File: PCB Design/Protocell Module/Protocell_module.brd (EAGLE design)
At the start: 70.8 x 27.9 mm, 19 parts, among them IC1 MC7805BDTRKG, X3 RJ45-8X

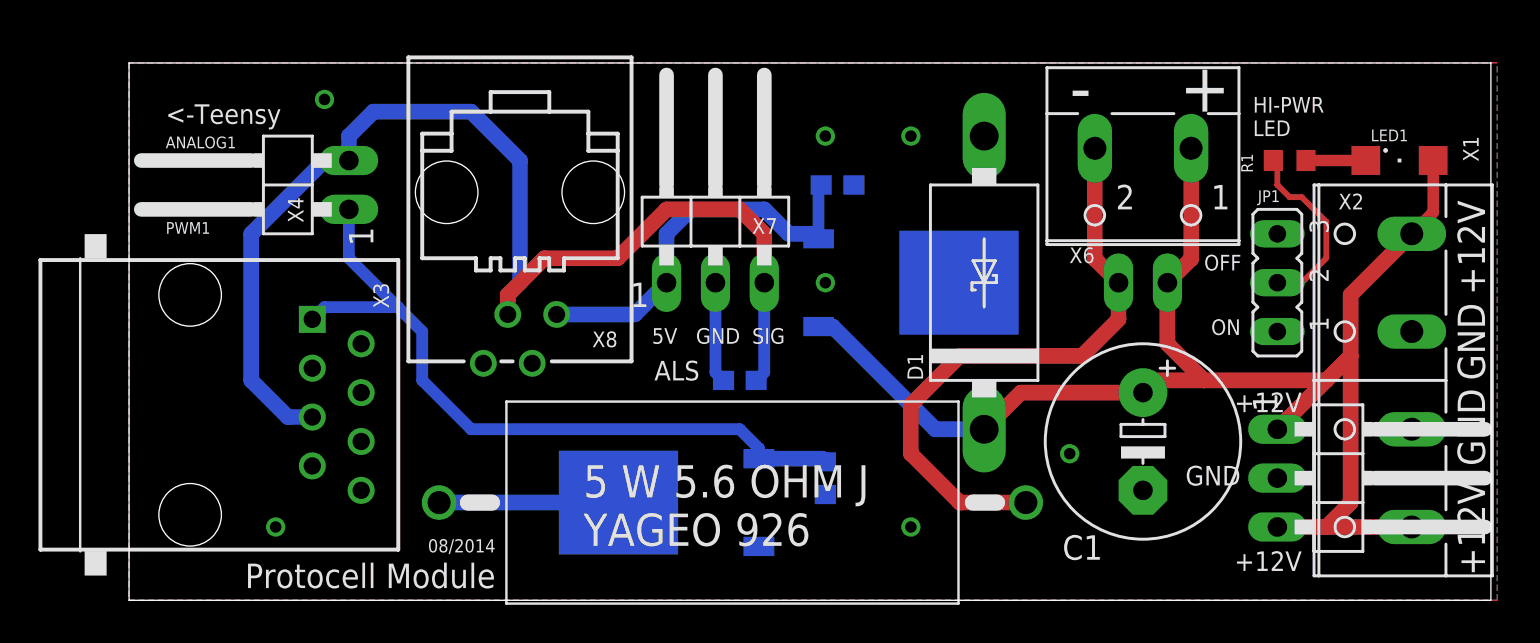
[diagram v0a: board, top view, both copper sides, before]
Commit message: Generated gerber files
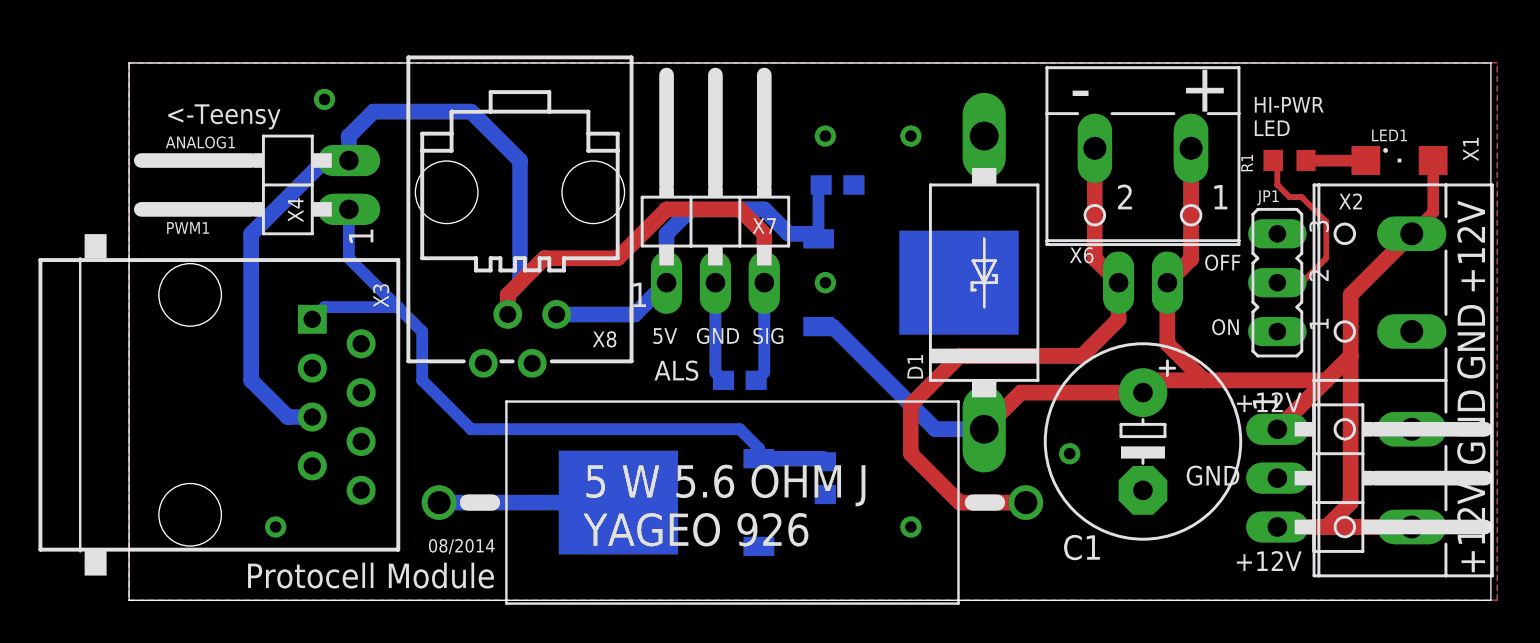
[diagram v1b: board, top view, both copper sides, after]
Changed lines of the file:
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@@
 </class>
 </classes>
-<designrules name="default *">
-<description language="de">&lt;b&gt;EAGLE Design Rules&lt;/b&gt;
-&lt;p&gt;
-Die Standard-Design-Rules sind so gewählt, dass sie für
-die meisten Anwendungen passen. Sollte ihre Platine
-besondere Anforderungen haben, treffen Sie die erforderlichen
-Einstellungen hier und speichern die Design Rules unter
-einem neuen Namen ab.</description>
+<designrules name="SparkFun">
 <description language="en">&lt;b&gt;EAGLE Design Rules&lt;/b&gt;
 &lt;p&gt;
@@
 <param name="mtCopper" value="0.035mm 0.035mm 0.035mm 0.035mm 0.035mm 0.035mm 0.035mm 0.035mm 0.035mm 0.035mm 0.035mm 0.035mm 0.035mm 0.035mm 0.035mm 0.035mm"/>
 <param name="mtIsolate" value="1.5mm 0.15mm 0.2mm 0.15mm 0.2mm 0.15mm 0.2mm 0.15mm 0.2mm 0.15mm 0.2mm 0.15mm 0.2mm 0.15mm 0.2mm"/>
-<param name="mdWireWire" value="10mil"/>
-<param name="mdWirePad" value="10mil"/>
-<param name="mdWireVia" value="10mil"/>
-<param name="mdPadPad" value="10mil"/>
-<param name="mdPadVia" value="10mil"/>
-<param name="mdViaVia" value="10mil"/>
+<param name="mdWireWire" value="8mil"/>
+<param name="mdWirePad" value="8mil"/>
+<param name="mdWireVia" value="8mil"/>
+<param name="mdPadPad" value="8mil"/>
+<param name="mdPadVia" value="8mil"/>
+<param name="mdViaVia" value="8mil"/>
 <param name="mdSmdPad" value="8mil"/>
 <param name="mdSmdVia" value="8mil"/>
@@
 <param name="mdViaViaSameLayer" value="8mil"/>
 <param name="mnLayersViaInSmd" value="2"/>
-<param name="mdCopperDimension" value="40mil"/>
+<param name="mdCopperDimension" value="10mil"/>
 <param name="mdDrill" value="8mil"/>
 <param name="mdSmdStop" value="0mil"/>
-<param name="msWidth" value="10mil"/>
+<param name="msWidth" value="8mil"/>
 <param name="msDrill" value="20mil"/>
 <param name="msMicroVia" value="9.99mm"/>
@@
 <param name="rvMicroViaOuter" value="0.25"/>
 <param name="rvMicroViaInner" value="0.25"/>
-<param name="rlMinPadTop" value="10mil"/>
+<param name="rlMinPadTop" value="12mil"/>
 <param name="rlMaxPadTop" value="20mil"/>
 <param name="rlMinPadInner" value="10mil"/>
 <param name="rlMaxPadInner" value="20mil"/>
-<param name="rlMinPadBottom" value="10mil"/>
+<param name="rlMinPadBottom" value="12mil"/>
 <param name="rlMaxPadBottom" value="20mil"/>
-<param name="rlMinViaOuter" value="8mil"/>
+<param name="rlMinViaOuter" value="10mil"/>
 <param name="rlMaxViaOuter" value="20mil"/>
-<param name="rlMinViaInner" value="8mil"/>
+<param name="rlMinViaInner" value="10mil"/>
 <param name="rlMaxViaInner" value="20mil"/>
 <param name="rlMinMicroViaOuter" value="4mil"/>
@@
 <param name="mlMinCreamFrame" value="0mil"/>
 <param name="mlMaxCreamFrame" value="0mil"/>
-<param name="mlViaStopLimit" value="0mil"/>
+<param name="mlViaStopLimit" value="25mil"/>
 <param name="srRoundness" value="0"/>
 <param name="srMinRoundness" value="0mil"/>
